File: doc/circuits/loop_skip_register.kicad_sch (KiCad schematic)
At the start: 12 parts, among them U1 74LS193, U10 74LS32, U11 74LS32, U12 74LS04, U13 74LS193, U3 74LS245, U4 74LS04, U5 74LS04, U6 74LS32, U7 74LS245, U8 74LS32, U9 74LS32

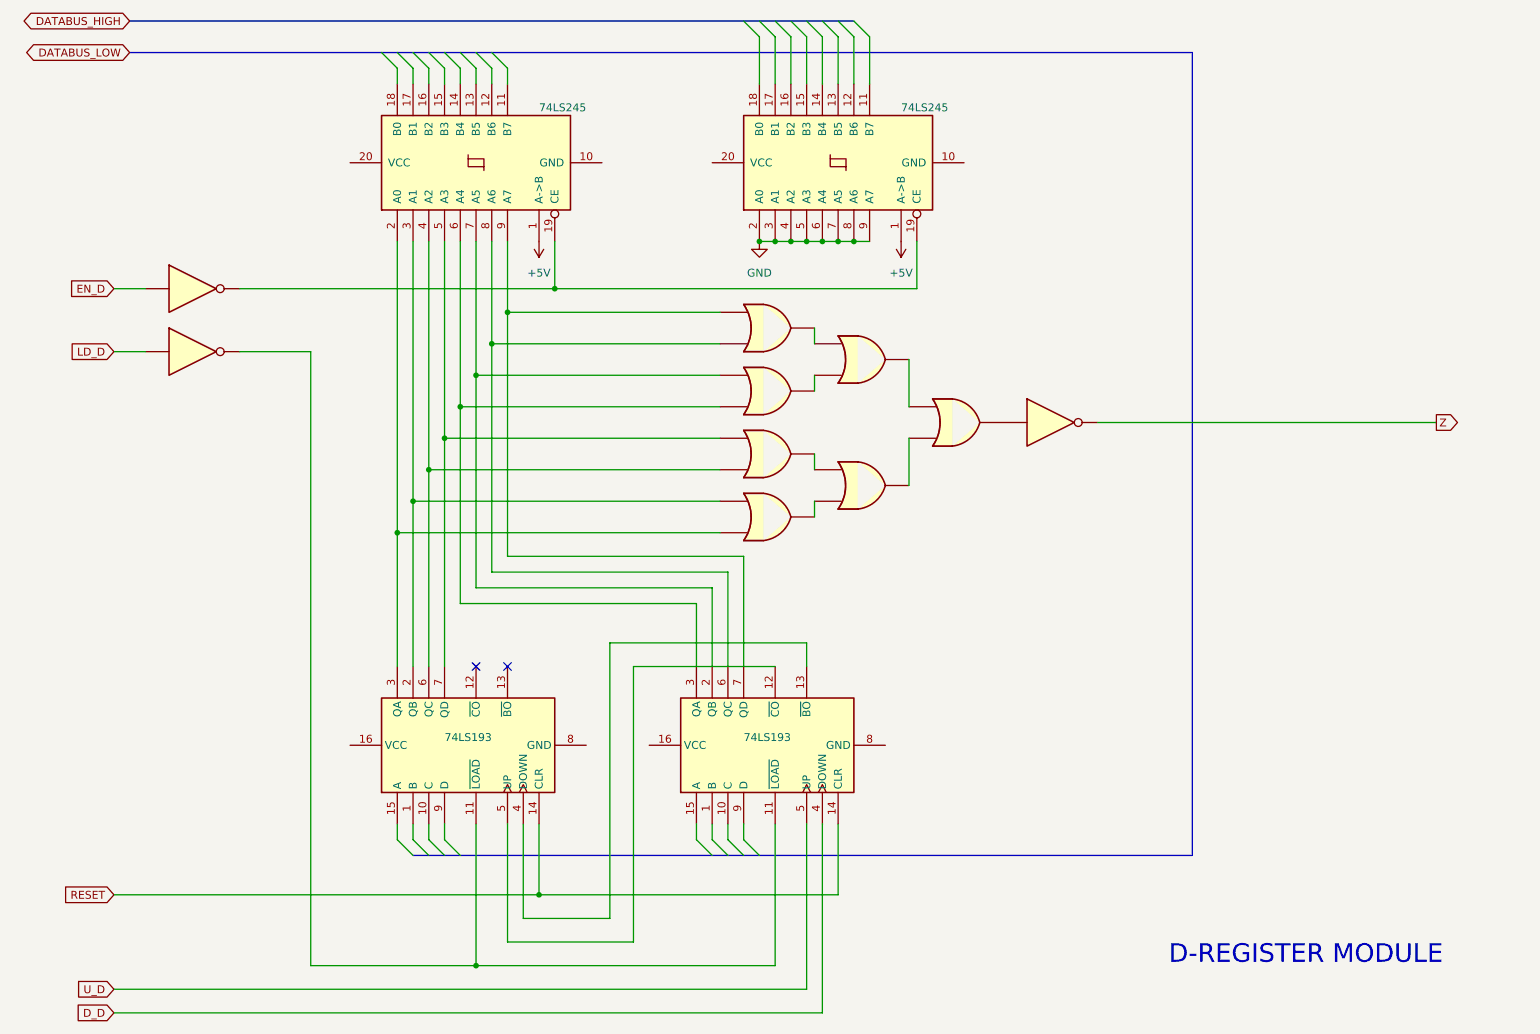
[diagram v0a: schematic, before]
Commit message: Updated schematics
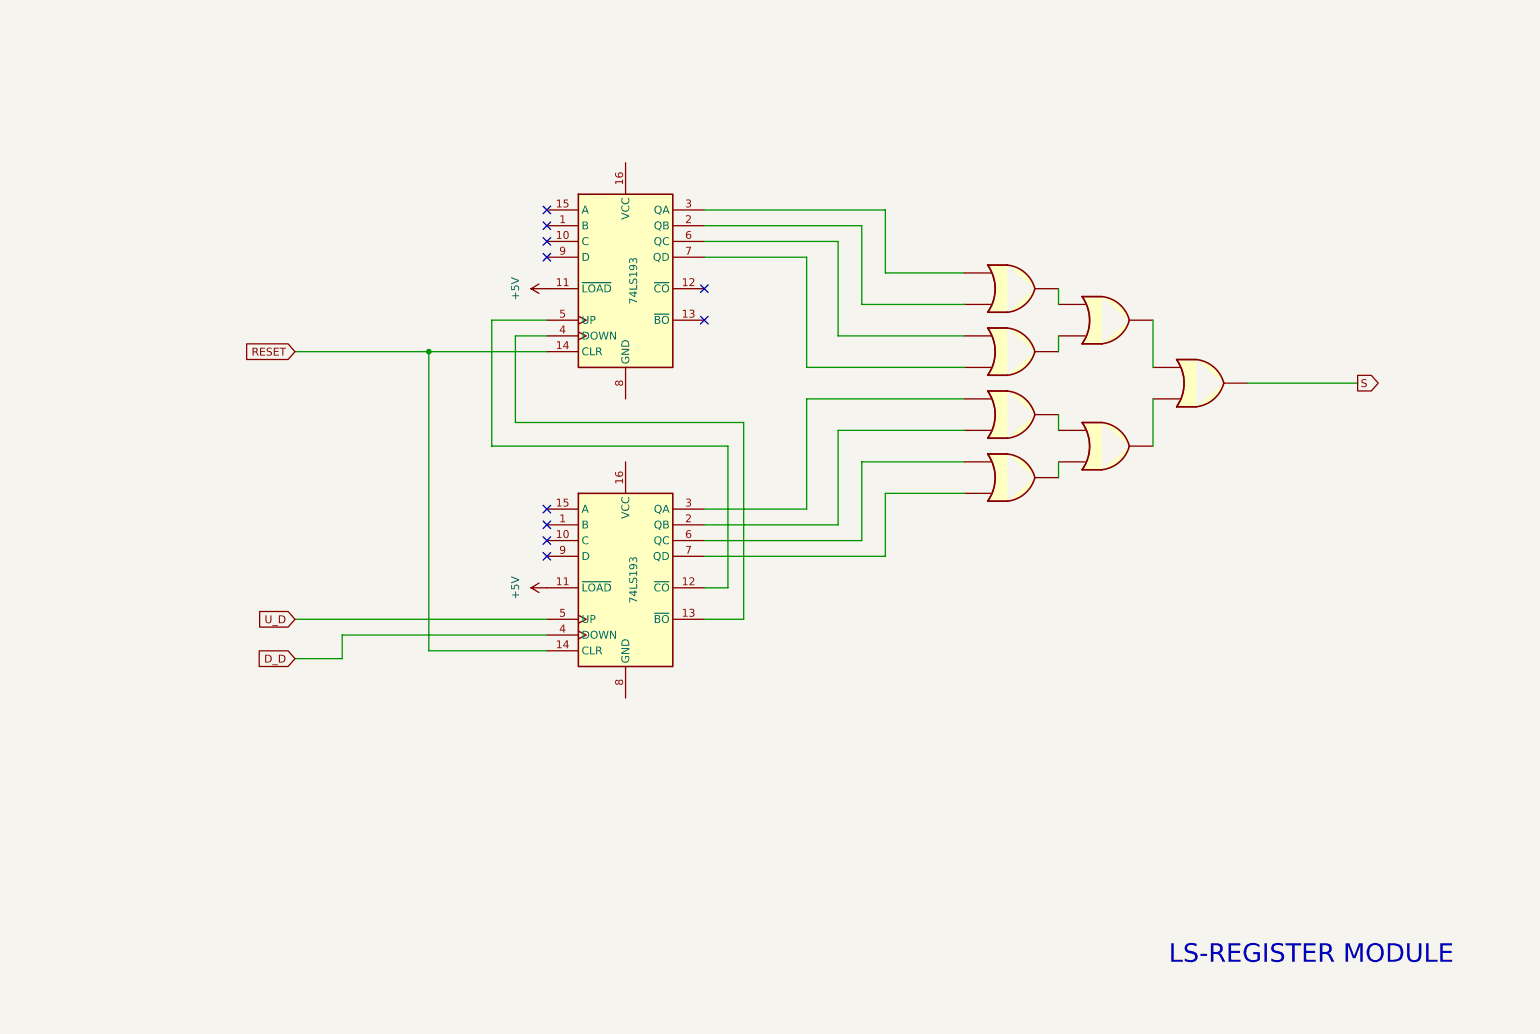
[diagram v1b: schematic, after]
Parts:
- removed U12, U4, U5: 74LS04, symbol 74xx:74LS04
- removed U3, U7: 74LS245, symbol 74xx:74LS245
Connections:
- net +5V: now also U1.11 (~{LOAD}), U13.11 (~{LOAD})
- net at U1.3 (QA): now also U6.1; no longer U9.5
- net at U1.2 (QB): now also U6.2; no longer U9.4
- net at U1.6 (QC): now also U6.4; no longer U9.2
- net at U1.7 (QD): now also U6.5; no longer U9.1
- net at U13.3 (QA): now also U9.1; no longer U6.5
- net at U13.2 (QB): now also U9.2; no longer U6.4
- net at U13.6 (QC): now also U9.4; no longer U6.2
- net at U13.7 (QD): now also U9.5; no longer U6.1
- net S: now reaches U11.3
- no-connect marks 2 -> 10
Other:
- note added: "LS-REGISTER MODULE"
- note removed: "D-REGISTER MODULE"
